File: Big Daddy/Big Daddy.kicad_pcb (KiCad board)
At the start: 4 copper layers, 245.5 x 127 mm, 127 parts, among them J1 JST-B2B-VERT-2PIN, J10 Conn_01x02, J11 Conn_01x23, J12 Conn_01x14, J13 Conn_01x14, J15 Conn_01x02, J2 JST-B2B-VERT-2PIN, J3 HV+, J4 HV-, J5 GND, J6 HV+, J7 HV-, J8 Conn_01x14, J9 Conn_01x08, K1 T9VV1K15-12S, K2 G5V-2, K3 G5V-2, K4 J107, K5 G5V-1, Q1 2N7002, Q2 BCP53, Q3 IXFH34N65X2, Q4 IXFH34N65X2, Q6 MMBT2222, U1 MAX33054EASA+T, U10 TLP184, U11 LM5050-1, U12 LM5050-1, U14 LM317_TO-263, U2 ESP32-S3-DevKitC, U3 ESP32-S3-DevKitC, U4 LT1528CQ#PBF, U5 LTV-817S, U6 ICM7555xB, U7 IS31LT3360, U8 Vicor_AERO, U9 LTV-817S

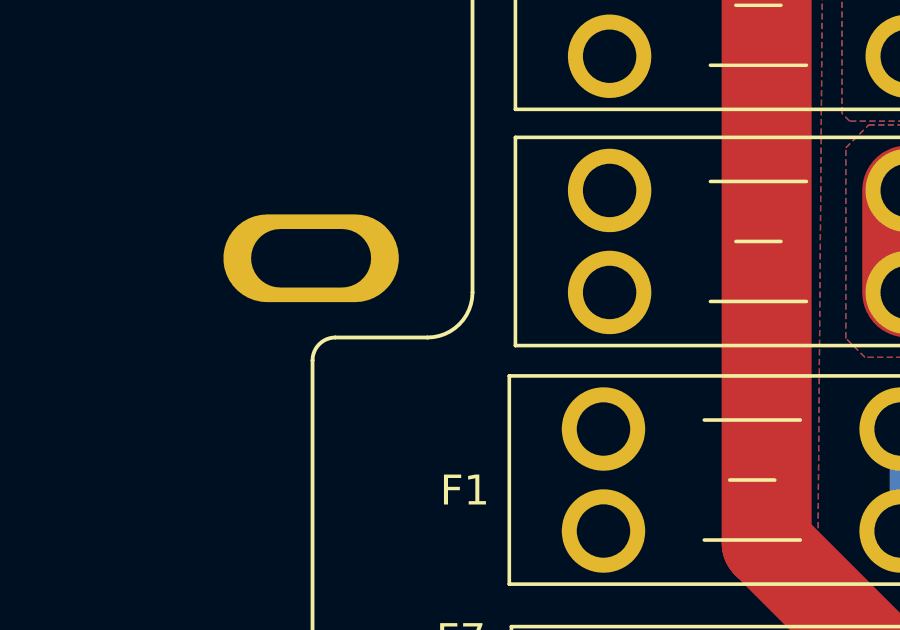
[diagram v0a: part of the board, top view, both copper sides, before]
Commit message: post comp
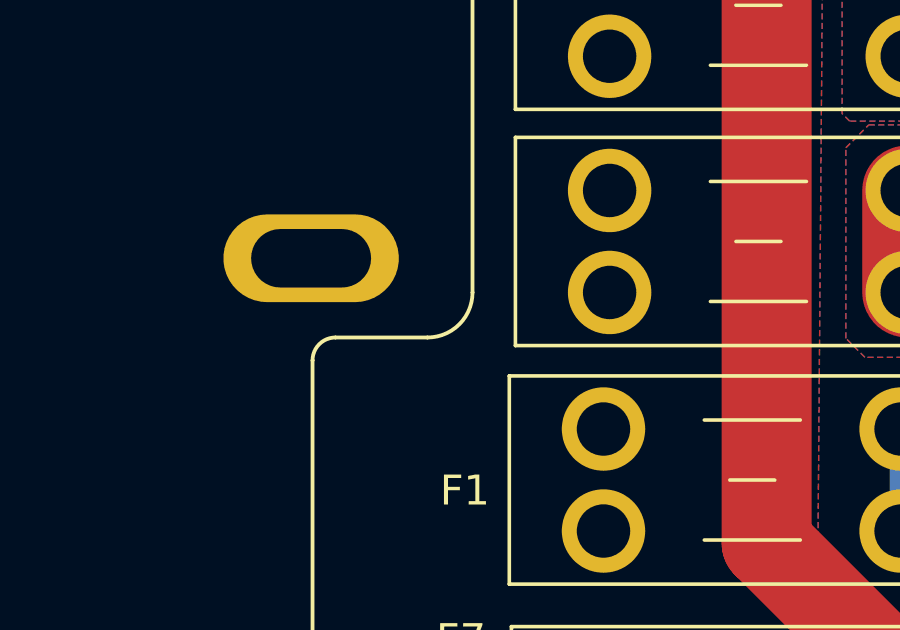
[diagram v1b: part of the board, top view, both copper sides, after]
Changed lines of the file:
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@@
     (fp_arc (start 13.254599 -13.5891) (mid 14.315331 -13.149731) (end 14.7547 -12.089)
       (stroke (width 0.127) (type solid)) (layer "F.SilkS"))
-    (fp_arc (start 14.755 -2.289221) (mid 14.315485 -1.228417) (end 13.2546 -0.789094)
+    (fp_arc (start 14.755 -2.289221) (mid 14.315486 -1.228414) (end 13.2546 -0.789094)
       (stroke (width 0.127) (type solid)) (layer "F.SilkS"))
     (fp_line (start -12.925 2.51078) (end -12.925 -12.089)
@@
     (fp_arc (start 13.2546 -13.8391) (mid 14.492108 -13.326508) (end 15.0047 -12.089)
       (stroke (width 0.05) (type solid)) (layer "F.CrtYd"))
-    (fp_arc (start 15.005 -2.28922) (mid 14.492262 -1.05164) (end 13.2546 -0.539094)
+    (fp_arc (start 15.005 -2.28922) (mid 14.492262 -1.051637) (end 13.2546 -0.539094)
       (stroke (width 0.05) (type solid)) (layer "F.CrtYd"))
     (fp_line (start -12.675 2.51078) (end -12.675 -12.089)
@@
     (fp_arc (start 13.254599 -13.5891) (mid 14.315331 -13.149731) (end 14.7547 -12.089)
       (stroke (width 0.127) (type solid)) (layer "F.Fab"))
-    (fp_arc (start 14.755 -2.289221) (mid 14.315485 -1.228417) (end 13.2546 -0.789094)
+    (fp_arc (start 14.755 -2.289221) (mid 14.315486 -1.228414) (end 13.2546 -0.789094)
       (stroke (width 0.127) (type solid)) (layer "F.Fab"))
     (fp_circle (center -5.08 0) (end -4.7625 0)
